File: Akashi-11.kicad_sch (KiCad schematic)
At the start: 2 parts, among them CN10 PPPC192LFBN-RC, CN7 PPPC192LFBN-RC

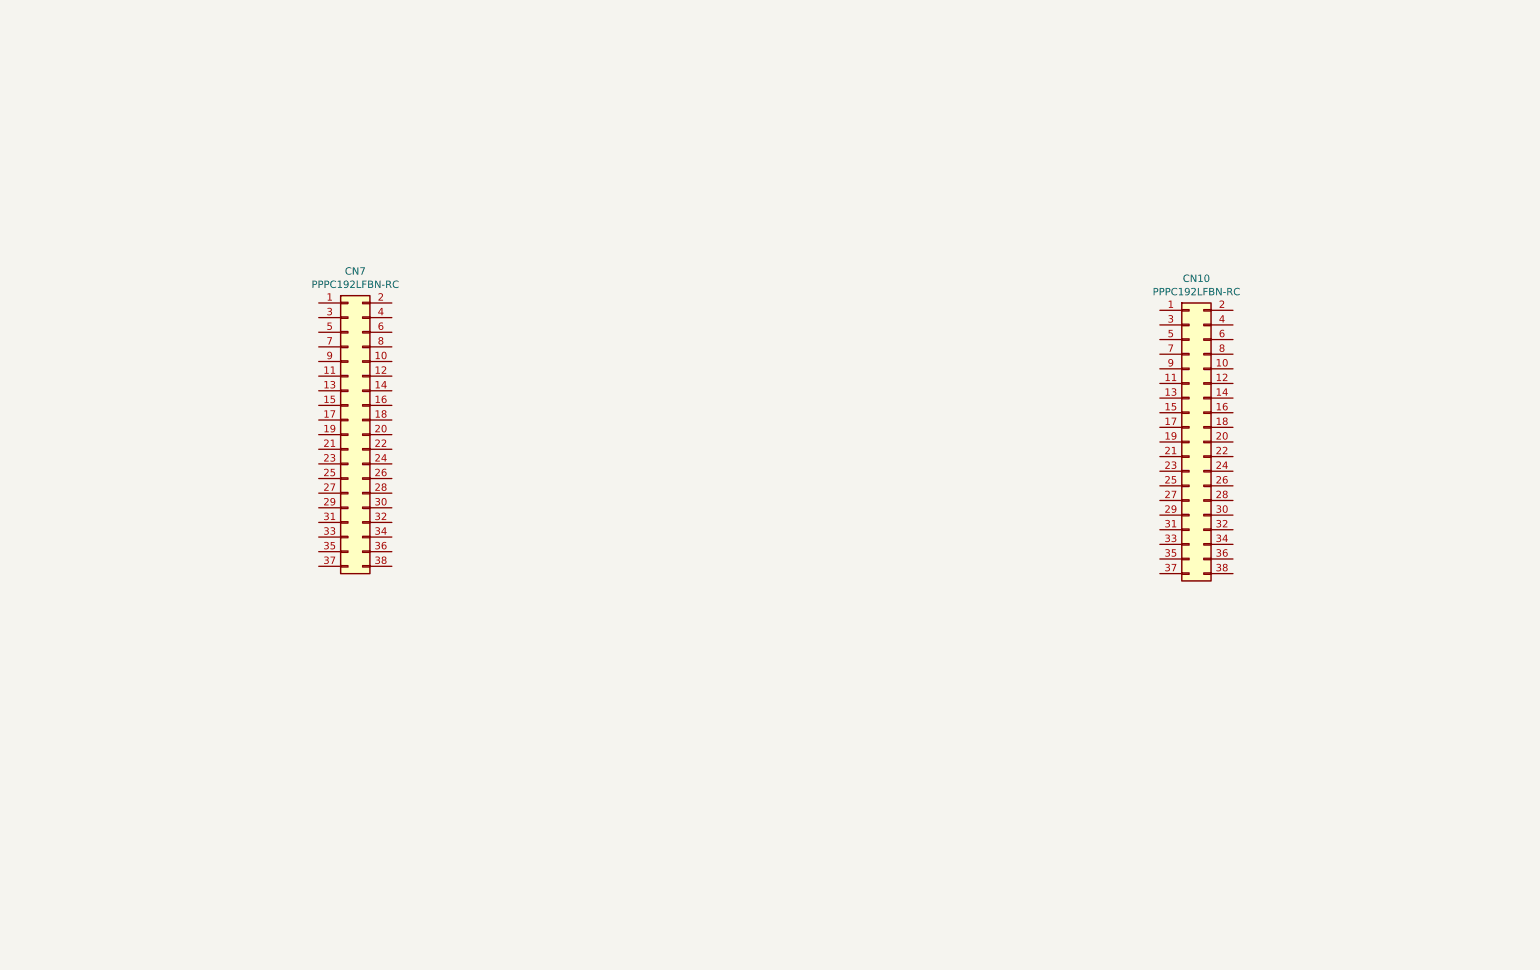
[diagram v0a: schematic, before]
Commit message: Rough schematics drawing.
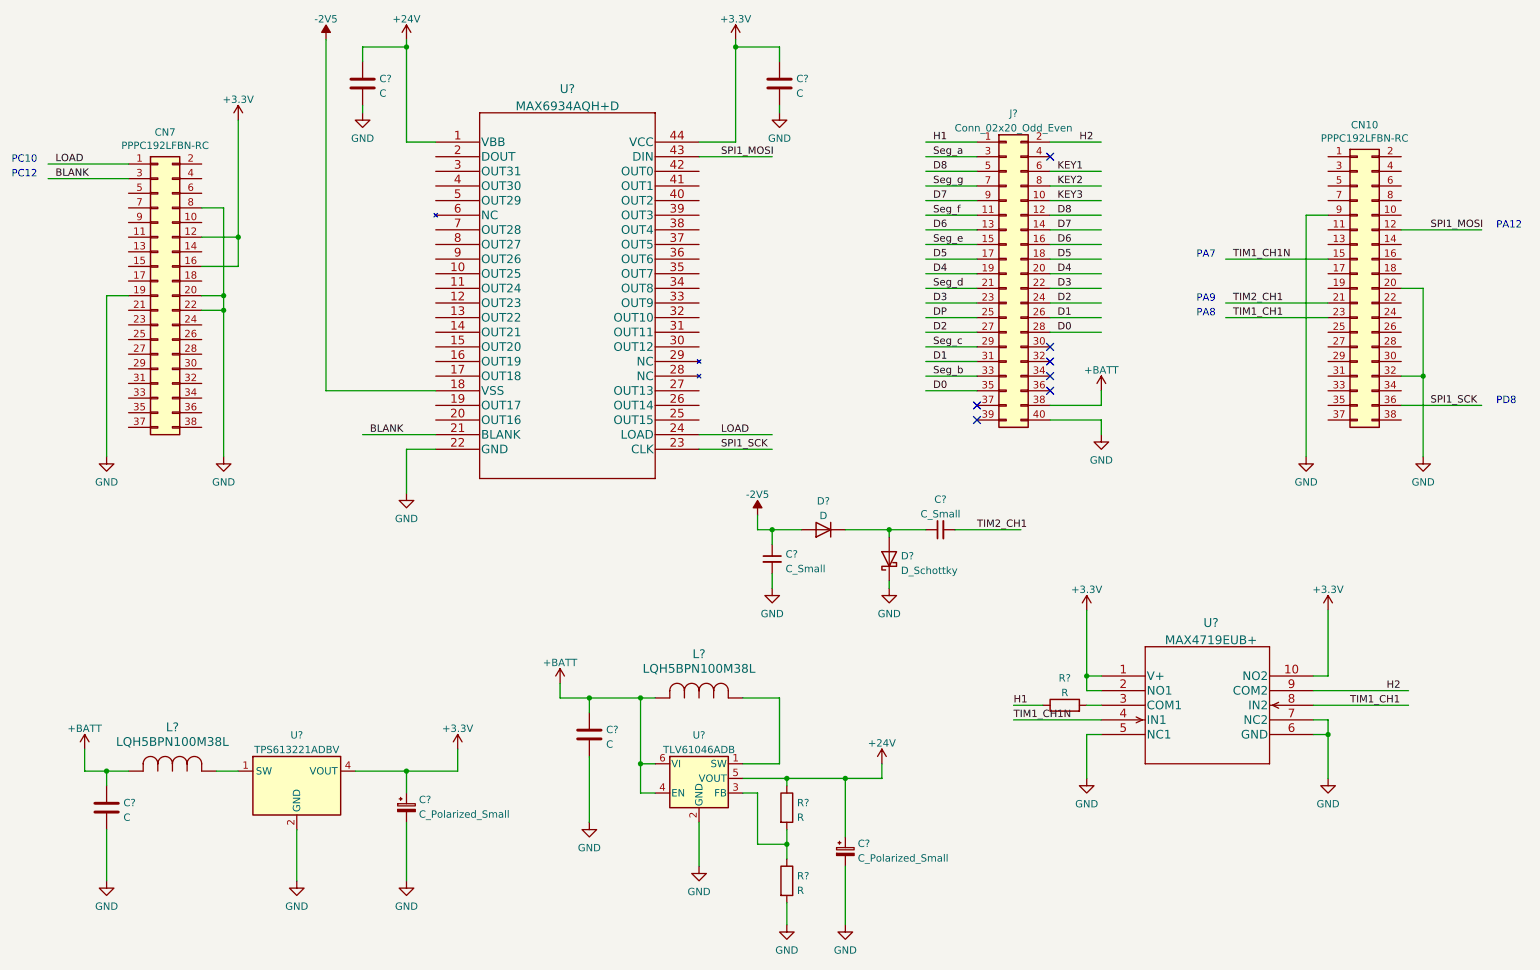
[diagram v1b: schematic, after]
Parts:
- added C? (x4): C, symbol Device:C
- added C? (x2): C_Small, symbol Device:C_Small
- added C? (x2): C_Polarized_Small, symbol Device:C_Polarized_Small
- added D?: D_Schottky, symbol Device:D_Schottky
- added D?: D, symbol Device:D
- added J?: Conn_02x20_Odd_Even, symbol Connector_Generic:Conn_02x20_Odd_Even
- added L? (x2): LQH5BPN100M38L, IND_LQH5BPN_MUR, symbol LQH5BPN100M:LQH5BPN100M38L
- added R? (x3): R, symbol Device:R
- added U?: TPS613221ADBV, Package_TO_SOT_SMD:SOT-23-5, symbol Regulator_Switching:TPS613221ADBV
- added U?: TLV61046ADB, Package_TO_SOT_SMD:SOT-23-6, symbol Regulator_Switching:TLV61046ADB
- added U?: MAX6934AQH+D, 21-0049_Q44+1_MXM, symbol MA6934AQH:MAX6934AQH+D
- added U?: MAX4719EUB+, 21-0061L, symbol MAX4719EUB:MAX4719EUB+
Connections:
- net LOAD: now reaches CN7.1 (Pin_1)
- net LOAD: now also U?.24 (LOAD)
- net +3V3: now reaches CN7.12 (Pin_12)
- net +3V3: now also CN7.16 (Pin_16), C?.1, C?.1, U?.1 (V+), U?.10 (NO2), U?.2 (NO1), U?.4 (VOUT), U?.44 (VCC)
- net GND: now reaches CN7.19 (Pin_19)
- net GND: now also CN10.20 (Pin_20), CN10.32 (Pin_32), CN10.9 (Pin_9), CN7.20 (Pin_20), CN7.22 (Pin_22), CN7.8 (Pin_8), C?.2, C?.2, C?.2, C?.2, C?.2, C?.2, C?.2, D?.1 (K), J?.40 (Pin_40), R?.2, U?.2 (GND), U?.2 (GND), U?.22 (GND), U?.5 (NC1), U?.6 (GND), U?.7 (NC2)
- net BLANK: now reaches CN7.3 (Pin_3)
- net BLANK: now also U?.21 (BLANK)
- net SPI1_MOSI: now reaches CN10.12 (Pin_12)
- net SPI1_MOSI: now also U?.43 (DIN)
- net TIM1_CH1N: now reaches CN10.15 (Pin_15)
- net TIM1_CH1N: now also U?.4 (IN1)
- net TIM2_CH1: now reaches CN10.21 (Pin_21)
- net TIM2_CH1: now also C?.2
- net TIM1_CH1: now reaches CN10.23 (Pin_23)
- net TIM1_CH1: now also U?.8 (IN2)
- net SPI1_SCK: now reaches CN10.36 (Pin_36)
- net SPI1_SCK: now also U?.23 (CLK)
- new net: L?.1, U?.1 (SW) (x2)
- new net: R?.1, R?.2, U?.3 (FB)
- new net: C?.1, D?.1 (K), D?.2 (A)
- new net: R?.2, U?.3 (COM1)
- new net +24V: C?.1, C?.1, R?.1, U?.1 (VBB), U?.5 (VOUT)
- new net +BATT: C?.1, C?.1, J?.38 (Pin_38), L?.2, L?.2, U?.4 (EN), U?.6 (VI)
- new net -2V5: C?.1, D?.2 (A), U?.18 (VSS)
- new net D0: J?.28 (Pin_28), J?.35 (Pin_35)
- new net D1: J?.26 (Pin_26), J?.31 (Pin_31)
- new net D2: J?.24 (Pin_24), J?.27 (Pin_27)
- new net D3: J?.22 (Pin_22), J?.23 (Pin_23)
- new net D4: J?.19 (Pin_19), J?.20 (Pin_20)
- new net D5: J?.17 (Pin_17), J?.18 (Pin_18)
- new net D6: J?.13 (Pin_13), J?.16 (Pin_16)
- new net D7: J?.14 (Pin_14), J?.9 (Pin_9)
- new net D8: J?.12 (Pin_12), J?.5 (Pin_5)
- new net DP: J?.25 (Pin_25)
- new net H1: J?.1 (Pin_1), R?.1
- new net H2: J?.2 (Pin_2), U?.9 (COM2)
- new net KEY1: J?.6 (Pin_6)
- new net KEY2: J?.8 (Pin_8)
- new net KEY3: J?.10 (Pin_10)
- new net Seg_a: J?.3 (Pin_3)
- new net Seg_b: J?.33 (Pin_33)
- new net Seg_c: J?.29 (Pin_29)
- new net Seg_d: J?.21 (Pin_21)
- new net Seg_e: J?.15 (Pin_15)
- new net Seg_f: J?.11 (Pin_11)
- new net Seg_g: J?.7 (Pin_7)
- no-connect marks 0 -> 7
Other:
- note added: "PA12"
- note added: "PA7"
- note added: "PA8"
- note added: "PA9"
- note added: "PC10"
- note added: "PC12"
- note added: "PD8"
- moved on the sheet: CN10, CN7
